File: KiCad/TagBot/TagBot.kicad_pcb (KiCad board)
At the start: 4 copper layers, 54 x 57 mm, 81 parts, among them IC101 ADXL343BCCZ-RL, J1001 Conn_01x06, J1002 Conn_01x06, J101 Conn_ST_STDC14, J103 Conn_01x03, J105 Conn_01x02, J1101 Conn_01x04, J801 Conn_01x06, J901 Conn_01x08, SW701 SW_Push, SW702 SW_Push, U101 STM32G431CBUx, U201 ZXBM5210-SP, U301 ZXBM5210-SP, U401 MP1475S, U501 BU33SD5WG-TR, Y101 Crystal

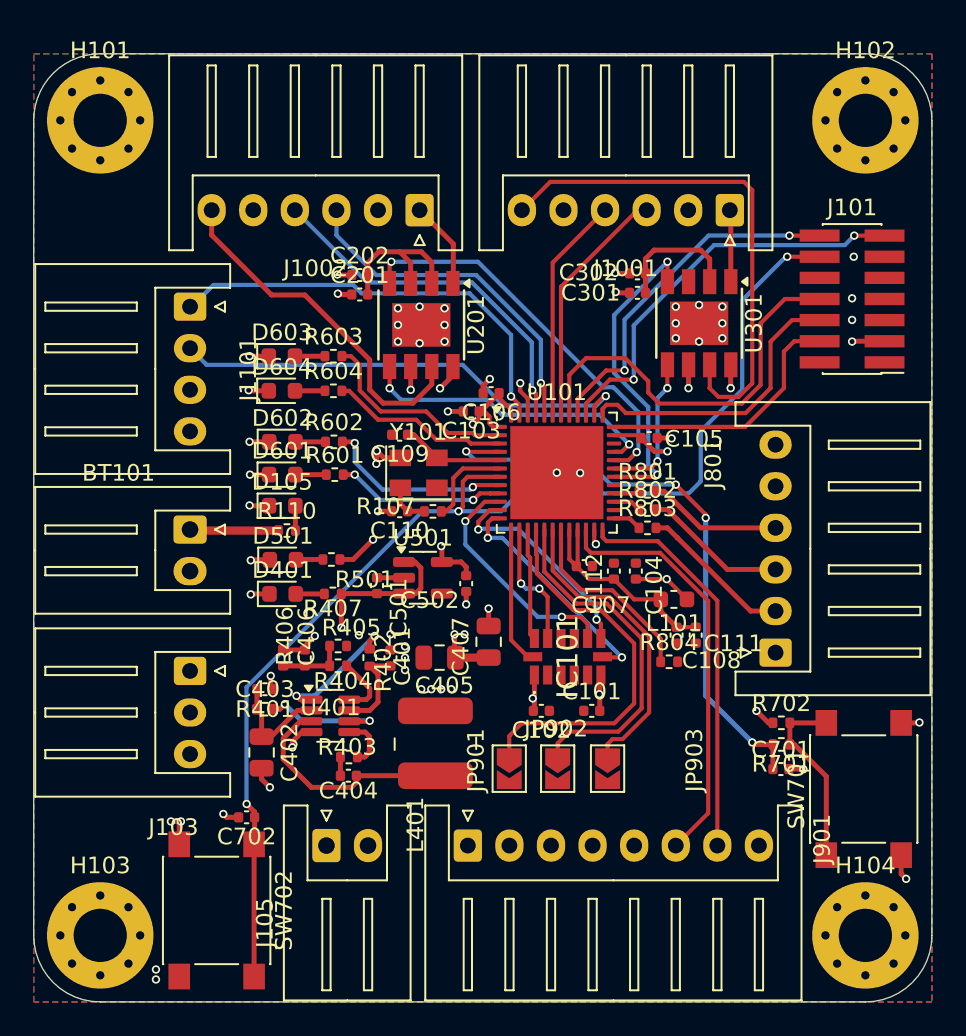
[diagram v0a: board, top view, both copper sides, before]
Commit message: update routage
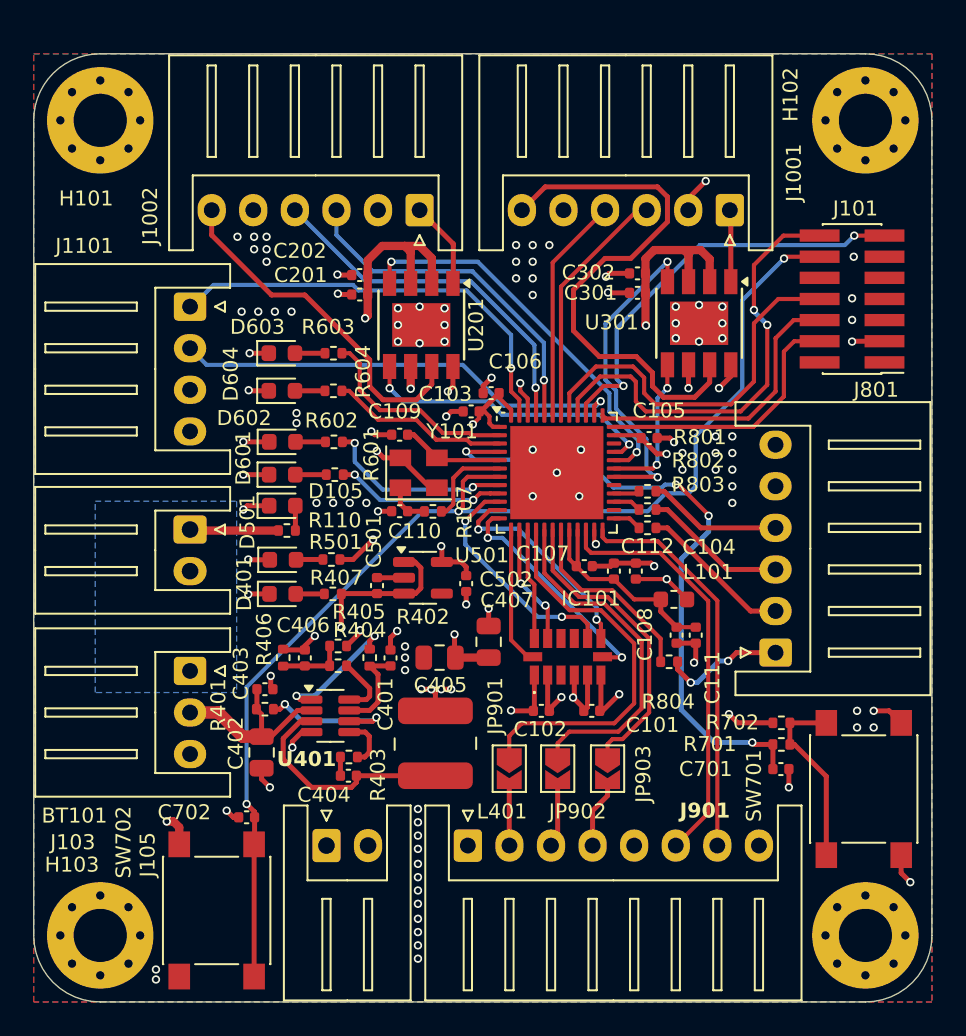
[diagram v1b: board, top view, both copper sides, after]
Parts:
- moved D603 0.18 mm to (50.9, 54.0)
- moved R603 0.18 mm to (54.0, 54.0)
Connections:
- J1101 pad 3: +5V -> +3.3V
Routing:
- net +3.3V: track 27.6 -> 78.9 mm
- net GND: track 36.8 -> 63.9 mm, vias 59 -> 115
- net Net-(J103-Pin_3): track 0.00 -> 12.5 mm
- net /Valim: track 26.8 -> 38.0 mm, vias 2 -> 4
- net Net-(J801-Pin_1): track 0.00 -> 7.42 mm, vias 0 -> 2
- net /STLINK_RX: track 21.4 -> 27.4 mm
- net Net-(J901-Pin_4): track 0.00 -> 4.27 mm
- net Net-(J901-Pin_3): track 0.00 -> 4.07 mm
- net Net-(J901-Pin_2): track 0.00 -> 3.90 mm
- net +5V: track 15.2 -> 18.4 mm, vias 8 -> 7
- net /BTN_CAT_MOUSE: track 35.6 -> 38.6 mm
- net /RIGHT_OUT2: track 30.9 -> 32.6 mm
- net /SYS_JTDO-SWO: track 24.2 -> 23.2 mm
- net Net-(U401-EN/SYNC): track 7.56 -> 8.53 mm
- net /OLED_SCL: track 28.1 -> 27.2 mm
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- added copper zone on In2.Cu, net /Valim
- added copper zone on B.Cu, net /Vbatterie
